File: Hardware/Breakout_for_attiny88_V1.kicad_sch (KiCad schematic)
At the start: 14 parts, among them J1 Conn_01x08, J2 Conn_01x08, J3 Conn_01x08, J4 AVR-ISP-6, J5 Conn_01x02, J6 Conn_01x02, SW1 SW, U1 ATtiny88

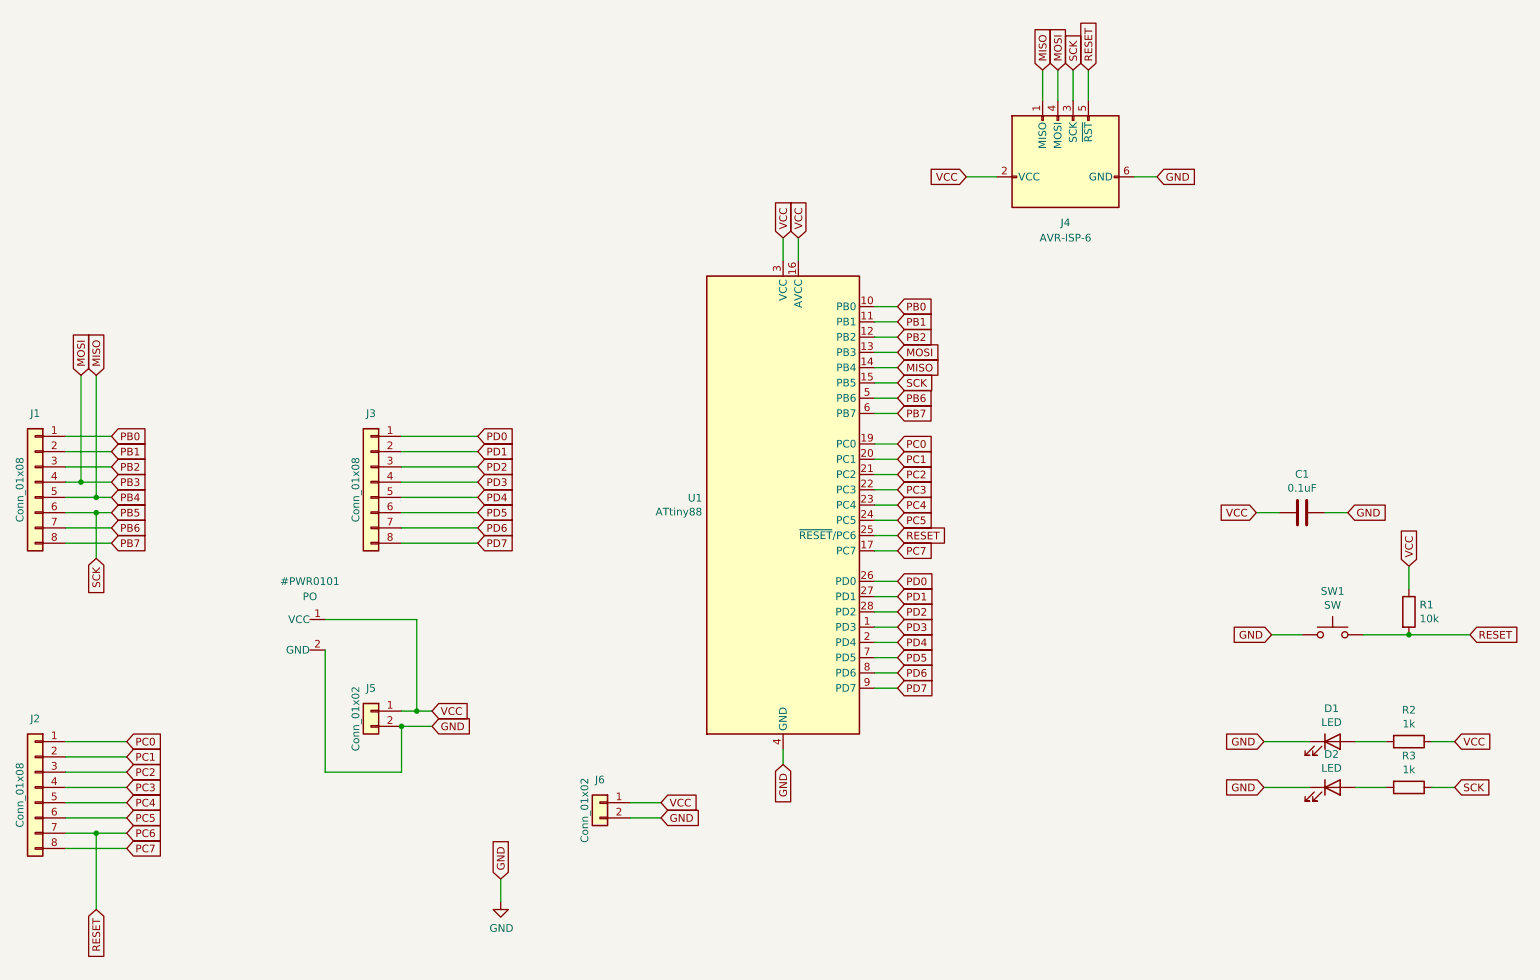
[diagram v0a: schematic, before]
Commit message: Added_New_PCB
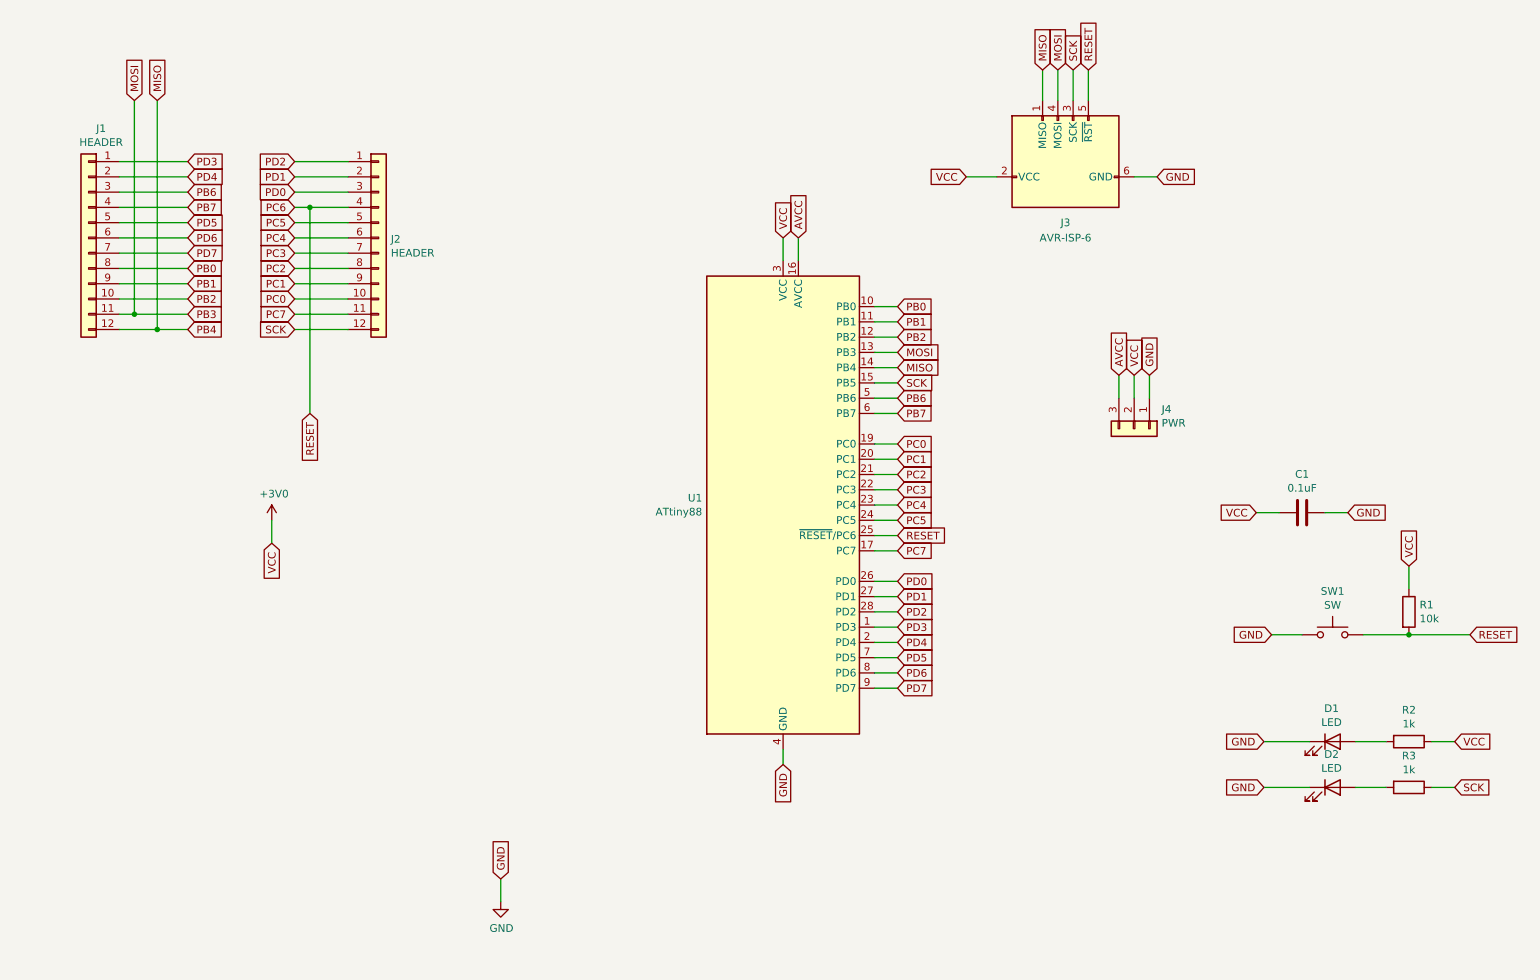
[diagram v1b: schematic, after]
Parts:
- removed J1, J2, J3: Conn_01x08, Connector_PinHeader_2.54mm:PinHeader_1x08_P2.54mm_Vertical, symbol Connector_Generic:Conn_01x08
- removed J5, J6: Conn_01x02, Connector_PinHeader_2.54mm:PinHeader_1x02_P2.54mm_Vertical, symbol Connector_Generic:Conn_01x02
- added J1, J2: HEADER, Pin_Headers:Pin_Header_Straight_1x12_Pitch2.54mm, symbol Connector_Generic:Conn_01x12
- added J4: PWR, Pin_Headers:Pin_Header_Straight_1x03_Pitch2.54mm, symbol Connector_Generic:Conn_01x03
- J3: renamed from J4; footprint Connector_PinHeader_2.54mm:PinHeader_2x03_P2.54mm_Vertical -> Connector_IDC:IDC-Header_2x03_P2.54mm_Vertical
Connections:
- net GND: now also J4.1 (Pin_1)
- net MISO: now also J1.12 (Pin_12)
- net MOSI: now also J1.11 (Pin_11)
- net PB0: now also J1.8 (Pin_8)
- net PB1: now also J1.9 (Pin_9)
- net PB2: now also J1.10 (Pin_10)
- net PB6: now also J1.3 (Pin_3)
- net PB7: now also J1.4 (Pin_4)
- net PC0: now also J2.10 (Pin_10)
- net PC1: now also J2.9 (Pin_9)
- net PC2: now also J2.8 (Pin_8)
- net PC3: now also J2.7 (Pin_7)
- net PC4: now also J2.6 (Pin_6)
- net PC5: now also J2.5 (Pin_5)
- net PC6: now also J2.4 (Pin_4)
- net PC7: now also J2.11 (Pin_11)
- net PD0: now also J2.3 (Pin_3)
- net PD1: now also J2.2 (Pin_2)
- net PD2: now also J2.1 (Pin_1)
- net PD3: now also J1.1 (Pin_1)
- net PD4: now also J1.2 (Pin_2)
- net PD5: now also J1.5 (Pin_5)
- net PD6: now also J1.6 (Pin_6)
- net PD7: now also J1.7 (Pin_7)
- net PB5 renamed SCK
- net SCK: now also J2.12 (Pin_12)
- net VCC renamed +3V0
- net +3V0: now also J4.2 (Pin_2); no longer U1.16 (AVCC)
- new net AVCC: J4.3 (Pin_3), U1.16 (AVCC)
